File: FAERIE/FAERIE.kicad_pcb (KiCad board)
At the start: 2 copper layers, 43.4 x 93 mm, 41 parts, among them J1 UV Sensor, J10 12V IN, J11 Batt IN, J2 UV Bulb, J3 Sparkmax PWM, J4 Sparkmax, J5 Laser1, J7 CAN, J8 CAM1, J9 CAM2, Q1 SSM3K329R_LF, U1 D24V22Fx, U2 TJA1051T-3

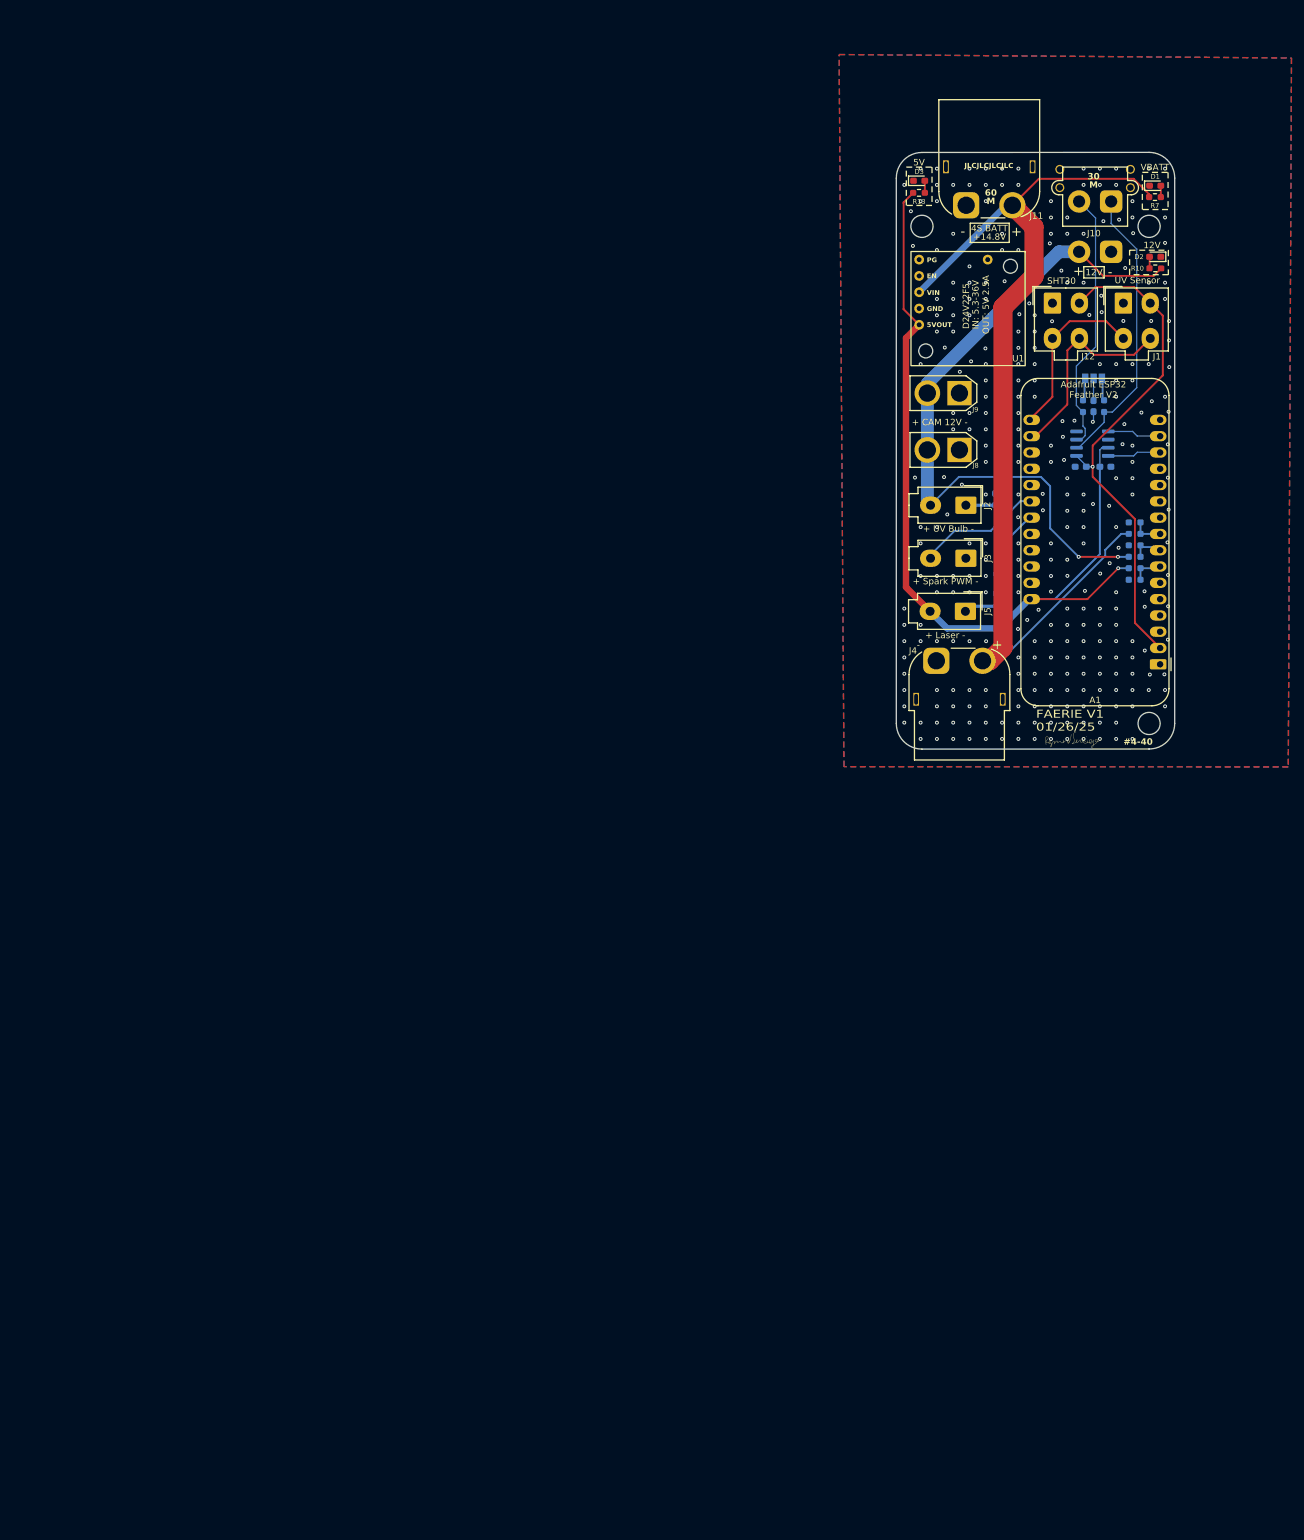
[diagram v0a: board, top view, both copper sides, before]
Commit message: FAERIE 2026 V1
FAERIE April 15, 2026
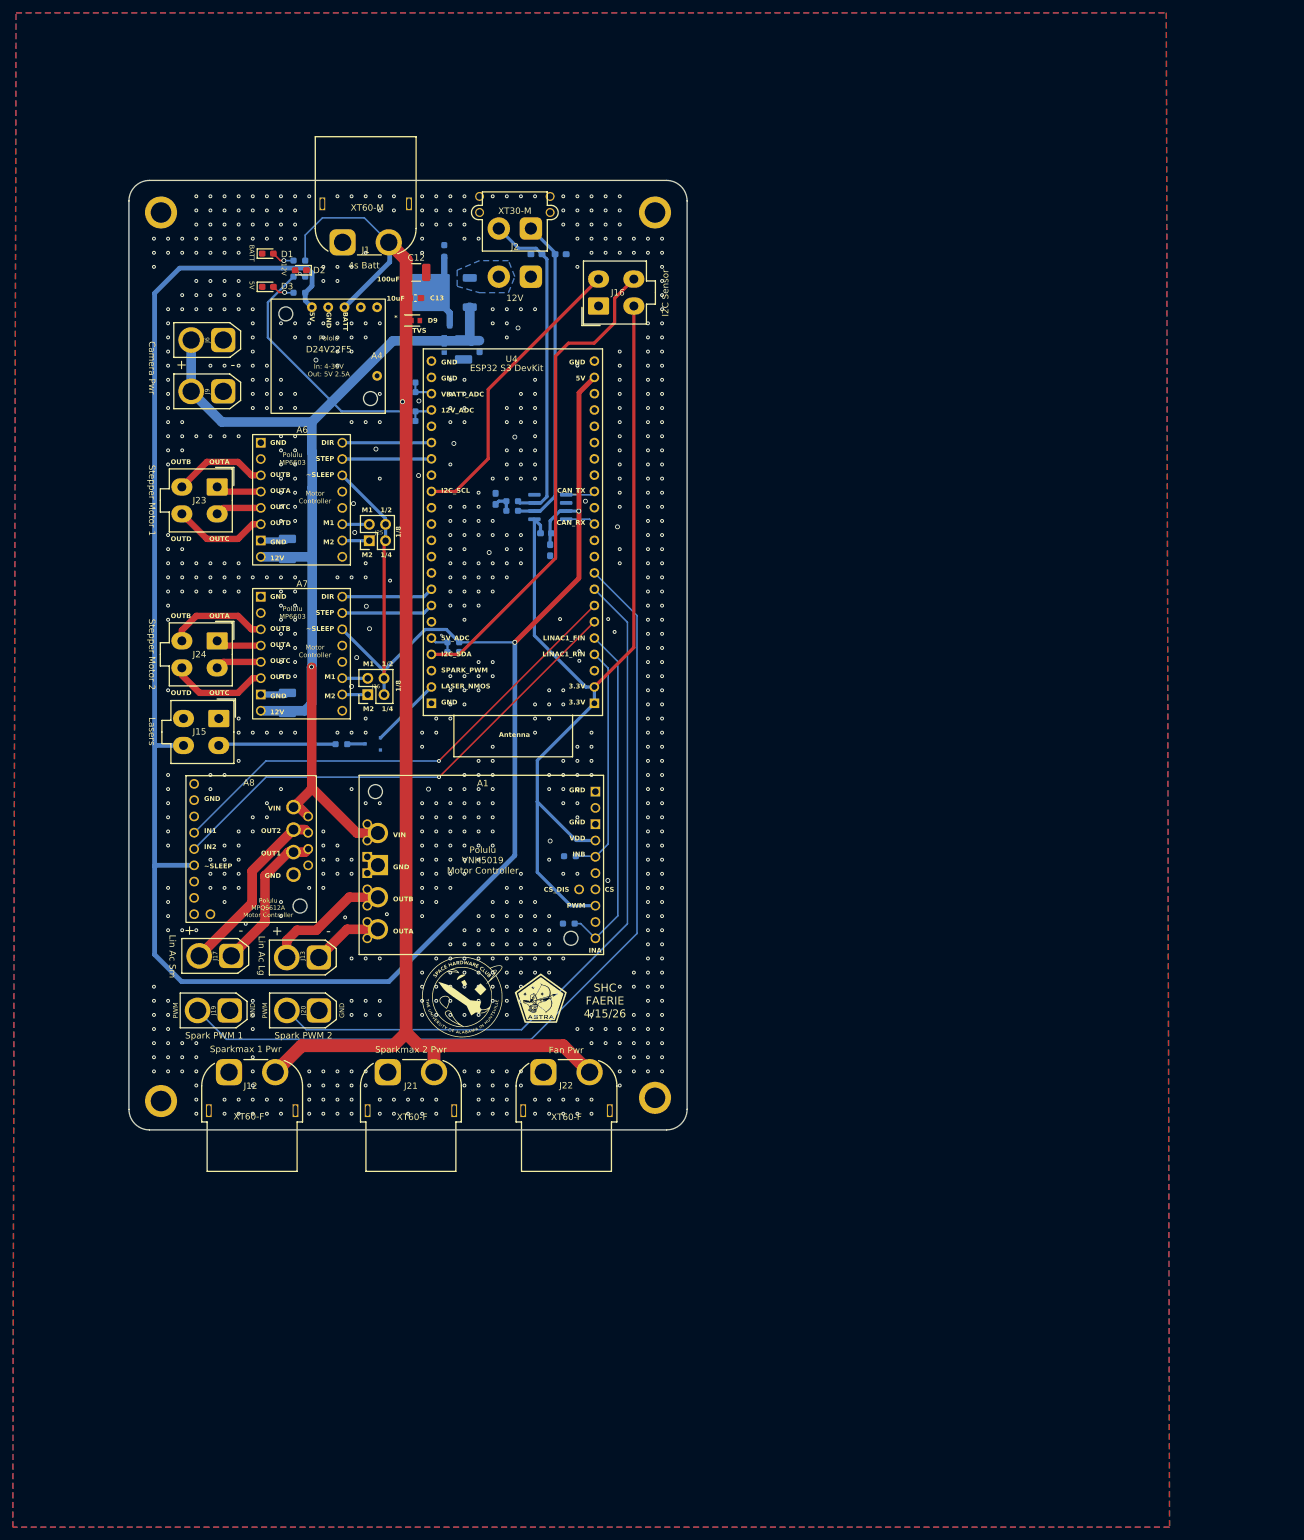
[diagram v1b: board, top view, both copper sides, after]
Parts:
- removed the G*** at (180.3, 128.9)
- removed the G*** at (181.6, 121.0)
- removed the G*** at (182.3, 108.6)
- removed J10: 12V IN, Connector_AMASS:AMASS_XT30PW-M_1x02_P2.50mm_Horizontal
- removed J11: Batt IN, Connector_AMASS:AMASS_XT60PW-M_1x02_P7.20mm_Horizontal
- removed J4: Sparkmax, Connector_AMASS:AMASS_XT60PW-F_1x02_P7.20mm_Horizontal
- removed J5: Laser1, Connector_Molex:Molex_Mini-Fit_Jr_5566-02A_2x01_P4.20mm_Vertical
- removed J7: CAN, Connector_AMASS:AMASS_XT30PW-F_1x02_P2.50mm_Horizontal
- removed J8: CAM1, Core_fp:XT30M_MODIFIED
- removed JP1: SolderJumper_3_Open, Jumper:SolderJumper-3_P1.3mm_Open_Pad1.0x1.5mm_NumberLabels
- removed Q1: SSM3K329R_LF, Core_fp:SOTFL95P240X88-3N
- removed R1: 60, Resistor_SMD:R_0603_1608Metric_Pad0.98x0.95mm_HandSolder
- removed R13: R_5V, Resistor_SMD:R_0603_1608Metric_Pad0.98x0.95mm_HandSolder
- removed the REF** at (192.3, 125.8)
- removed the REF** at (156.9, 48.3)
- removed the REF** at (192.3, 48.3)
- removed SHT30: ~, Connector_Molex:Molex_Mini-Fit_Jr_5566-04A_2x02_P4.20mm_Vertical
- removed U2: TJA1051T-3, Package_SO:SOIC-8_3.9x4.9mm_P1.27mm
- added A4: D24V22F5, FAERIE:D24V22Fx, F.Cu at (73.2, 77.4)
- added A6: MP6603_5690, FAERIE:MP6603-5690, F.Cu at (67.8, 101.1)
- added A7: MP6603_5690, FAERIE:MP6603-5690, F.Cu at (67.8, 125.1)
- added A8: MPQ6612A_5285, FAERIE:MPQ6612A_5285, F.Cu at (42.2, 133.9)
- added C12: 100uF, Capacitor_SMD:C_1210_3225Metric_Pad1.33x2.70mm_HandSolder, F.Cu at (78.1, 55.5)
- added C13: 10uF, Capacitor_SMD:C_0603_1608Metric_Pad1.08x0.95mm_HandSolder, F.Cu at (78.0, 59.5)
- added C14: 100uF, Capacitor_SMD:C_1210_3225Metric_Pad1.33x2.70mm_HandSolder, B.Cu at (58.0, 98.6)
- added C15: 100uF, Capacitor_SMD:C_1210_3225Metric_Pad1.33x2.70mm_HandSolder, B.Cu at (58.0, 122.6)
- added C4: 47 nF, Capacitor_SMD:C_0603_1608Metric_Pad1.08x0.95mm_HandSolder, B.Cu at (99.0, 98.8)
- added C5: 10uF, Capacitor_SMD:C_0603_1608Metric_Pad1.08x0.95mm_HandSolder, B.Cu at (88.0, 67.0)
- added C6: 100pF, Capacitor_SMD:C_0603_1608Metric_Pad1.08x0.95mm_HandSolder, B.Cu at (100.6, 52.6)
- added C7: 100pF, Capacitor_SMD:C_0603_1608Metric_Pad1.08x0.95mm_HandSolder, B.Cu at (96.8, 52.6)
- added D4: TVS, FAERIE:SOD-323HEUS2H_TOS, B.Cu at (82.5, 66.8)
- added D5: 15, Diode_SMD:D_SOD-123, B.Cu at (85.0, 63.6)
- added D9: TVS, FAERIE:SOD-323HEUS2H_TOS, F.Cu at (77.5, 63.0)
- added G***: SHC_Logo, FAERIE:SHC_Logo, F.Cu at (85.5, 168.5)
- added G***: ASTRA_Logo, FAERIE:ASTRA_Logo, F.Cu at (97.5, 168.5)
- added J12: Sparkmax 1 Pwr, Connector_AMASS:AMASS_XT60PW-F_1x02_P7.20mm_Horizontal, F.Cu at (48.9, 180.1)
- added J13: Lin Actuator 1 (Large), Connector_AMASS:AMASS_XT30U-F_1x02_P5.0mm_Vertical, F.Cu at (62.9, 162.3)
- added J15: Lasers, Connector_Molex:Molex_Mini-Fit_Jr_5566-04A_2x02_P4.20mm_Vertical, F.Cu at (47.3, 125.0)
- added J16: SHT30, Connector_Molex:Molex_Mini-Fit_Jr_5566-04A_2x02_P4.20mm_Vertical, F.Cu at (106.5, 60.7)
- added J17: Lin Actuator 2 (Small), Connector_AMASS:AMASS_XT30U-F_1x02_P5.0mm_Vertical, F.Cu at (49.2, 162.0)
- added J19: Sparkmax PWM 1, Connector_AMASS:AMASS_XT30U-F_1x02_P5.0mm_Vertical, F.Cu at (49.0, 170.5)
- added J20: Sparkmax PWM 2, Connector_AMASS:AMASS_XT30U-F_1x02_P5.0mm_Vertical, F.Cu at (62.9, 170.5)
- added J21: Sparkmax 2 Pwr, Connector_AMASS:AMASS_XT60PW-F_1x02_P7.20mm_Horizontal, F.Cu at (73.7, 180.1)
- added J22: Fan Pwr, Connector_AMASS:AMASS_XT60PW-F_1x02_P7.20mm_Horizontal, F.Cu at (97.9, 180.1)
- added J23: Stepper Motor 1, Connector_Molex:Molex_Mini-Fit_Jr_5566-04A_2x02_P4.20mm_Vertical, F.Cu at (47.0, 88.9)
- added J24: Stepper Motor 2, Connector_Molex:Molex_Mini-Fit_Jr_5566-04A_2x02_P4.20mm_Vertical, F.Cu at (47.0, 112.9)
- added J25: Stepper 1 Microstep Control, Connector_PinHeader_2.54mm:PinHeader_2x02_P2.54mm_Vertical, F.Cu at (70.8, 97.3)
- added J26: Stepper 2 Microstep Control, Connector_PinHeader_2.54mm:PinHeader_2x02_P2.54mm_Vertical, F.Cu at (70.5, 121.3)
- added J6: Cam 1 Pwr Conn, Connector_AMASS:AMASS_XT30U-F_1x02_P5.0mm_Vertical, F.Cu at (48.0, 66.0)
- added Q2: SSM3K329R_LF, FAERIE:SOT-23F_TOS, B.Cu at (71.3, 129.0)
- added Q3: PMOS, Package_TO_SOT_SMD:TO-252-2, B.Cu at (81.4, 58.6)
- added R17: 50k, Resistor_SMD:R_0603_1608Metric_Pad0.98x0.95mm_HandSolder, B.Cu at (82.5, 52.1)
- added R19: 0Ω, Resistor_SMD:R_0603_1608Metric_Pad0.98x0.95mm_HandSolder, B.Cu at (66.4, 129.0)
- added R20: 10k, Resistor_SMD:R_0603_1608Metric_Pad0.98x0.95mm_HandSolder, B.Cu at (102.0, 146.5)
- added R21: 10k, Resistor_SMD:R_0603_1608Metric_Pad0.98x0.95mm_HandSolder, B.Cu at (101.9, 157.0)
- added REF**: MountingHole_3.2mm_M3, MountingHole:MountingHole_3.2mm_M3, F.Cu at (38.3, 46.1)
- added REF**: MountingHole_3.2mm_M3, MountingHole:MountingHole_3.2mm_M3, F.Cu at (115.3, 46.1)
- added REF**: MountingHole_3.2mm_M3, MountingHole:MountingHole_3.2mm_M3, F.Cu at (38.3, 184.6)
- added REF**: MountingHole_3.2mm_M3, MountingHole:MountingHole_3.2mm_M3, F.Cu at (115.3, 184.1)
- added U4: ESP32 S3 DevKit, FAERIE:ESP32-S3-DevKit_No_Keep-Out_Zone, F.Cu at (107.1, 124.5)
- A1: value Adafruit Feather ESP32 V2 -> VNH5019_1451; footprint Module:Adafruit_Feather -> FAERIE:VNH5019_1451
- C1: value 100nF -> 4.7 nF
- C2: value 4.7nF -> 100uF; footprint Capacitor_SMD:C_0603_1608Metric_Pad1.08x0.95mm_HandSolder -> Capacitor_SMD:C_1210_3225Metric_Pad1.33x2.70mm_HandSolder
- C3: value 1 uF -> 100 nF
- D1: value VBATT -> BATT
- J1: value UV Sensor -> 4s Batt; footprint Connector_Molex:Molex_Mini-Fit_Jr_5566-04A_2x02_P4.20mm_Vertical -> Connector_AMASS:AMASS_XT60PW-M_1x02_P7.20mm_Horizontal
- J2: value UV Bulb -> 12V; footprint Connector_Molex:Molex_Mini-Fit_Jr_5566-02A_2x01_P4.20mm_Vertical -> Connector_AMASS:AMASS_XT30PW-M_1x02_P2.50mm_Horizontal
- J3: value Sparkmax PWM -> VIC CAN; footprint Connector_Molex:Molex_Mini-Fit_Jr_5566-02A_2x01_P4.20mm_Vertical -> Connector_AMASS:AMASS_XT30PW-F_1x02_P2.50mm_Horizontal; moved to B.Cu
- J9: value CAM2 -> CAM 2 Pwr Conn; footprint Core_fp:XT30M_MODIFIED -> Connector_AMASS:AMASS_XT30U-F_1x02_P5.0mm_Vertical
- R10: value R_12V -> R_5V; moved to B.Cu
- R11, R12: value 10 kΩ -> 60
- R2: value 60 -> 10k
- R3: value 330 -> 10k
- R4: value R_US -> R_BATT
- R5: value 10 kΩ -> 10k
- R6: value 3.1 kΩ -> 3.32k
- R7: value R_BATT -> 10k; moved to B.Cu
- R8: value 10 kΩ -> 2.21k
- R9: value 3.8 kΩ -> R_12V
- U1: value D24V22Fx -> TJA1051T/3; footprint Core_fp:D24V22Fx -> Package_SO:SOIC-8_3.9x4.9mm_P1.27mm; moved to B.Cu
- moved D1 138.7 mm to (55.0, 52.5)
- moved R9 136.8 mm to (59.9, 56.1), turned to 0 degrees
- moved R10 133.5 mm to (59.9, 58.6)
- moved D2 133.2 mm to (60.1, 55.1)
- moved J1 122.1 mm to (66.6, 50.8)
- moved R4 121.2 mm to (59.9, 53.6)
- moved R7 120.1 mm to (77.0, 74.1)
- moved R8 116.2 mm to (77.0, 72.6), turned to 180 degrees
- moved J9 114.8 mm to (48.0, 74.0)
- moved R5 114.6 mm to (77.0, 77.1)
- moved R6 114.1 mm to (77.0, 78.6)
- moved R2 107.9 mm to (83.9, 113.1), turned to 180 degrees
- moved D3 102.9 mm to (55.0, 57.7)
- moved C2 98.6 mm to (85.5, 67.5)
- moved A1 97.8 mm to (107.3, 161.8)
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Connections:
- A1 pad 1: unconnected-(A1-~{RESET}-Pad1) -> /LINAC1_FIN
- A1 pad 10: unconnected-(A1-IO_4/A5-Pad10) -> GND
- A1 pad 11: unconnected-(A1-SCK/IO5-Pad11) -> /LINAC1_NEG
- A1 pad 12: unconnected-(A1-MOSI/IO19-Pad12) -> /LINAC1_POS
- A1 pad 13: unconnected-(A1-MISO/IO21-Pad13) -> GND
- A1 pad 14: /RXTransceiver -> +12V
- A1 pad 15: /TXtransceiver -> unconnected-(A1-CS_DIS-Pad15)
- A1 pad 2: +3.3V -> unconnected-(A1-ENA/DIAGA-Pad2)
- A1 pad 3: unconnected-(A1-NC-Pad3) -> +3.3V
- A1 pad 4: GND -> unconnected-(A1-CS-Pad4)
- A1 pad 6: unconnected-(A1-IO25/A1-Pad6) -> /LINAC1_RIN
- A1 pad 7: /5V_ADC -> +3.3V
- A1 pad 8: /12V_ADC -> GND
- A1 pad 9: /BATT_ADC -> unconnected-(A1-VOUT-Pad9)
- C1 pad 1: +3.3V -> GND
- C1 pad 2: GND -> Net-(C1-Pad2)
- C2 pad 1: Net-(JP1-C) -> +12V
- C3 pad 2: GND -> +3.3V
- J1 pad 2: +3.3V -> +BATT
- J2 pad 1: Net-(J2-Pin_1) -> GND
- J2 pad 2: +12V -> /12V_IN
- J3 pad 1: GND -> /CAN_L
- J3 pad 2: /Sparkmax_PWM__A5 -> /CAN_H
- R10 pad 1: +12V -> +5V
- R10 pad 2: Net-(D2-A) -> Net-(D3-A)
- R11 pad 1: +5V -> /CAN_H
- R11 pad 2: /5V_ADC -> Net-(C1-Pad2)
- R12 pad 1: /5V_ADC -> Net-(C1-Pad2)
- R12 pad 2: GND -> /CAN_L
- R2 pad 1: Net-(JP1-A) -> +5V
- R2 pad 2: /CAN_L -> /5V_ADC
- R3 pad 1: GND -> /5V_ADC
- R3 pad 2: Net-(J2-Pin_1) -> GND
- R4 pad 1: Net-(J5-Pin_1) -> +BATT
- R4 pad 2: Net-(Q1-Pad3) -> Net-(D1-A)
- R5 pad 1: +BATT -> +12V
- R5 pad 2: /BATT_ADC -> /12V_ADC
- R6 pad 1: /BATT_ADC -> /12V_ADC
- R7 pad 2: Net-(D1-A) -> /BATT_ADC
- R8 pad 1: +12V -> /BATT_ADC
- R8 pad 2: /12V_ADC -> GND
- R9 pad 1: /12V_ADC -> +12V
- R9 pad 2: GND -> Net-(D2-A)
- U1 pad 1: unconnected-(U1-PG-Pad1) -> /CAN_TX
- U1 pad 2: unconnected-(U1-EN-Pad2) -> GND
- U1 pad 3: +BATT -> +5V
- U1 pad 4: GND -> /CAN_RX
- U1 pad 5: +5V -> +3.3V
- U1 pad 6: GND -> /CAN_L
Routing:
- net +5V: track 136.6 -> 371.8 mm, vias 1 -> 2
- net /SPARK1_PWM: track 0.00 -> 136.2 mm
- net /SPARK2_PWM: track 0.00 -> 115.4 mm
- net +12V: track 107.9 -> 201.8 mm, vias 2 -> 1
- net /LINAC2_RIN: track 0.00 -> 77.1 mm, vias 0 -> 1
- net /LINAC2_FIN: track 0.00 -> 77.1 mm, vias 0 -> 1
- net /I2C_SDA: track 0.00 -> 76.5 mm
- net +3.3V: track 80.2 -> 151.0 mm, vias 1 -> 0
- net +BATT: track 152.5 -> 217.3 mm, vias 0 -> 1
- net /LINAC1_FIN: track 0.00 -> 53.9 mm
- net /I2C_SCL: track 0.00 -> 46.1 mm
- net /LINAC1_RIN: track 0.00 -> 36.4 mm
- net /I2C_SCL_18: track 32.3 -> 0.00 mm
- net /LINAC2_POS: track 0.00 -> 28.3 mm
- net /I2C_SDA_17: track 27.4 -> 0.00 mm
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- added copper zone on B.Cu, net /12V_IN
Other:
- board size 43.4 x 93 mm -> 87 x 148 mm
- rule pad_to_mask_clearance: 0 -> 0.038
- board text added: "*"
- board text added: "0Ω"
- board text added: "1/2"
- board text added: "1/4"
- board text added: "1/8"
- board text added: "100 nF"
- board text added: "100uF"
- board text added: "10k"
- board text added: "10uF"
- board text added: "12V_ADC"
- board text added: "2.21k"
- board text added: "3.32k"
- board text added: "3.3V"
- board text added: "3V3"
- board text added: "47 nF"
- board text added: "4s Batt"
- board text added: "50k"
- board text added: "5V_ADC"
- board text added: "Antenna"
- board text added: "CAN_RX"
- board text added: "CAN_TX"
- board text added: "CS"
- board text added: "CS_DIS"
- board text added: "Cam 1"
- board text added: "Cam 2"
- board text added: "Camera Pwr"
- board text added: "D24V22F5 5V Buck"
- board text added: "DIR"
- board text added: "ESP32 S3 DevKit"
- board text added: "FAERIE ASTRA, SHC at UAH 87 x 148 mm"
- board text added: "Fan Pwr"
- board text added: "I2C Sensor"
- board text added: "I2C_SCL"
- board text added: "I2C_SDA"
- board text added: "IN1"
- board text added: "IN2"
- board text added: "INA"
- board text added: "INB"
- board text added: "In: 4-36V Out: 5V 2.5A"
- board text added: "LASER_NMOS"
- board text added: "LINAC1_FIN"
- board text added: "LINAC1_RIN"
- board text added: "Laser"
- board text added: "Lasers"
- board text added: "Lin Ac Lg"
- board text added: "Lin Ac Sm"
- board text added: "M1"
- board text added: "M2"
- board text added: "Motor Controller"
- board text added: "NEG"
- board text added: "NMOS"
- board text added: "OUT1"
- board text added: "OUT2"
- board text added: "OUTA"
- board text added: "OUTB"
- board text added: "OUTC"
- board text added: "OUTD"
- board text added: "PJD60P04E-AU"
- board text added: "POS"
- board text added: "PWM"
- board text added: "Pololu"
- board text added: "Polulu MP6603"
- board text added: "Polulu MP6603 Motor Controller"
- board text added: "Polulu MPQ6612A Motor Controller"
- board text added: "Polulu VNH5019 Motor Controller"
- board text added: "SHC FAERIE 4/15/26"
- board text added: "SPARK_PWM"
- board text added: "STEP"
- board text added: "Spark PWM 1"
- board text added: "Spark PWM 2"
- board text added: "Sparkmax 1 Pwr"
- board text added: "Sparkmax 2 Pwr"
- board text added: "Stepper 1"
- board text added: "Stepper 2"
- board text added: "Stepper Motor 1"
- board text added: "Stepper Motor 2"
- board text added: "TVS"
- board text added: "VBATT_ADC"
- board text added: "VDD"
- board text added: "Vic CAN"
- board text added: "XT30-M"
- board text added: "XT60-F"
- board text added: "XT60-M"
- board text added: "Zener"
- board text added: "{ "ViaStitching": "0.2", "GND": { "HSpacing": "1", "VSpacing": "1", "HOffset": "0", "VOffset": "0", "Clearance": "1", "Randomize": false } }"
- board text added: "{ "ViaStitching": "0.2", "GND": { "HSpacing": "1.27", "VSpacing": "1.27", "HOffset": "0", "VOffset": "0", "Clearance": "0.2", "Randomize": false } }"
- board text added: "{ "ViaStitching": "0.2", "GND": { "HSpacing": "2", "VSpacing": "2", "HOffset": "0", "VOffset": "0", "Clearance": "0.5", "Randomize": false } }"
- board text added: "{ "ViaStitching": "0.2", "GND": { "HSpacing": "2", "VSpacing": "2", "HOffset": "0", "VOffset": "0", "Clearance": "1", "Randomize": false } }"
- board text added: "{ "ViaStitching": "0.2", "GND": { "HSpacing": "2.2", "VSpacing": "2.2", "HOffset": "0", "VOffset": "0", "Clearance": "1", "Randomize": false } }"
- board text added: "{ "ViaStitching": "0.2", "GND": { "HSpacing": "2.5", "VSpacing": "2.5", "HOffset": "0", "VOffset": "0", "Clearance": ".25", "Randomize": false } }"
- board text added: "{ "ViaStitching": "0.2", "GND": { "HSpacing": "2.5", "VSpacing": "2.5", "HOffset": "0", "VOffset": "0", "Clearance": ".5", "Randomize": false } }"
- board text added: "{ "ViaStitching": "0.2", "GND": { "HSpacing": "2.5", "VSpacing": "2.5", "HOffset": "0", "VOffset": "0", "Clearance": "0.5", "Randomize": false } }"
- board text added: "{ "ViaStitching": "0.2", "GND": { "HSpacing": "2.5", "VSpacing": "2.5", "HOffset": "0", "VOffset": "0", "Clearance": "1", "Randomize": false } }"
- board text added: "{ "ViaStitching": "0.2", "GND": { "HSpacing": "3", "VSpacing": "3", "HOffset": "0", "VOffset": "0", "Clearance": ".5", "Randomize": false } }"
- board text added: "{ "ViaStitching": "0.2", "GND": { "HSpacing": "3", "VSpacing": "3", "HOffset": "0", "VOffset": "0", "Clearance": "0", "Randomize": false } }"
- board text added: "{ "ViaStitching": "0.2", "GND": { "HSpacing": "3", "VSpacing": "3", "HOffset": "0", "VOffset": "0", "Clearance": "1", "Randomize": false } }"
- board text added: "{ "ViaStitching": "0.2", "GND": { "HSpacing": "4", "VSpacing": "4", "HOffset": "0", "VOffset": "0", "Clearance": "1", "Randomize": false } }"
- board text added: "{ "ViaStitching": "0.2", "GND": { "HSpacing": "4", "VSpacing": "4", "HOffset": "0", "VOffset": "0", "Clearance": "4", "Randomize": false } }"
- board text added: "~SLEEP"
- board text removed: "#4-40"
- board text removed: "+ CAM 12V -"
- board text removed: "+ Laser -"
- board text removed: "+ Spark PWM -"
- board text removed: "+ UV Bulb -"
- board text removed: "+14.8V"
- board text removed: "+3.3V"
- board text removed: "0.1 μF"
- board text removed: "1.0 μF"
- board text removed: "10 kΩ"
- board text removed: "3.1 kΩ"
- board text removed: "3.8 kΩ"
- board text removed: "30"
- board text removed: "4S BATT"
- board text removed: "5VOUT"
- board text removed: "60"
- board text removed: "60Ω"
- board text removed: "Adafruit ESP32 Feather V2"
- board text removed: "CAN Transceiver"
- board text removed: "D"
- board text removed: "EN"
- board text removed: "F"
- board text removed: "FAERIE V1 01/26/25"
- board text removed: "Fouth Mounting 4-40 screw was deleted because of placemnet issues"
- board text removed: "G"
- board text removed: "IN: 5.3-36V OUT: 5V 2.5A"
- board text removed: "J12"
- board text removed: "JLCJLCJLCJLC"
- board text removed: "M"
- board text removed: "PG"
- board text removed: "S"
- board text removed: "SSM3K329R_LF"
- board text removed: "UV Sensor"
- board text removed: "VIC CAN"
